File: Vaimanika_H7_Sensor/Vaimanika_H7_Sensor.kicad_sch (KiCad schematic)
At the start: 67 parts, among them SW1 TS-1088-AR02016, U1 TCAN334G, U2 STM32H743VITx, U3 NCP163ASN330T1G, U4 MS5611-01BA, U5 ICM-42688-P, U6 ICM-42688-P, U7 W25Q128JVS, U8 RT9080-33GJ5, U9 BMI088, Y1 25 MHz

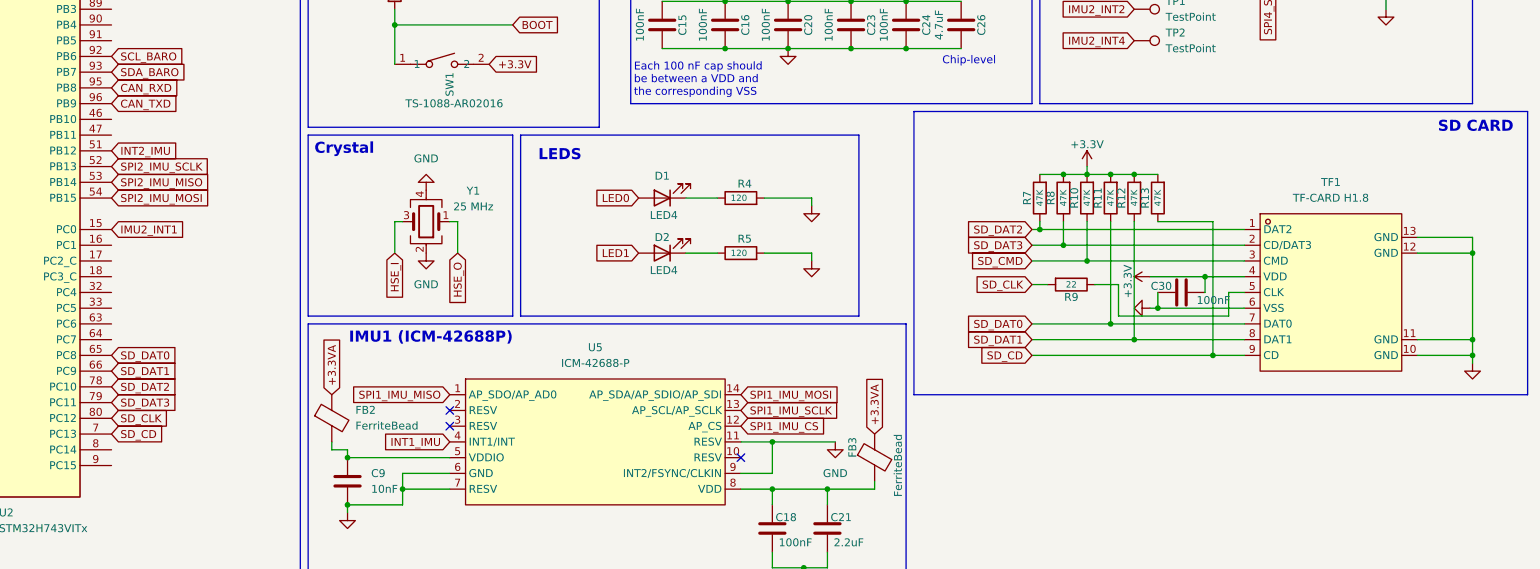
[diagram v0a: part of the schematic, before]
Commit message: 28-03-2025
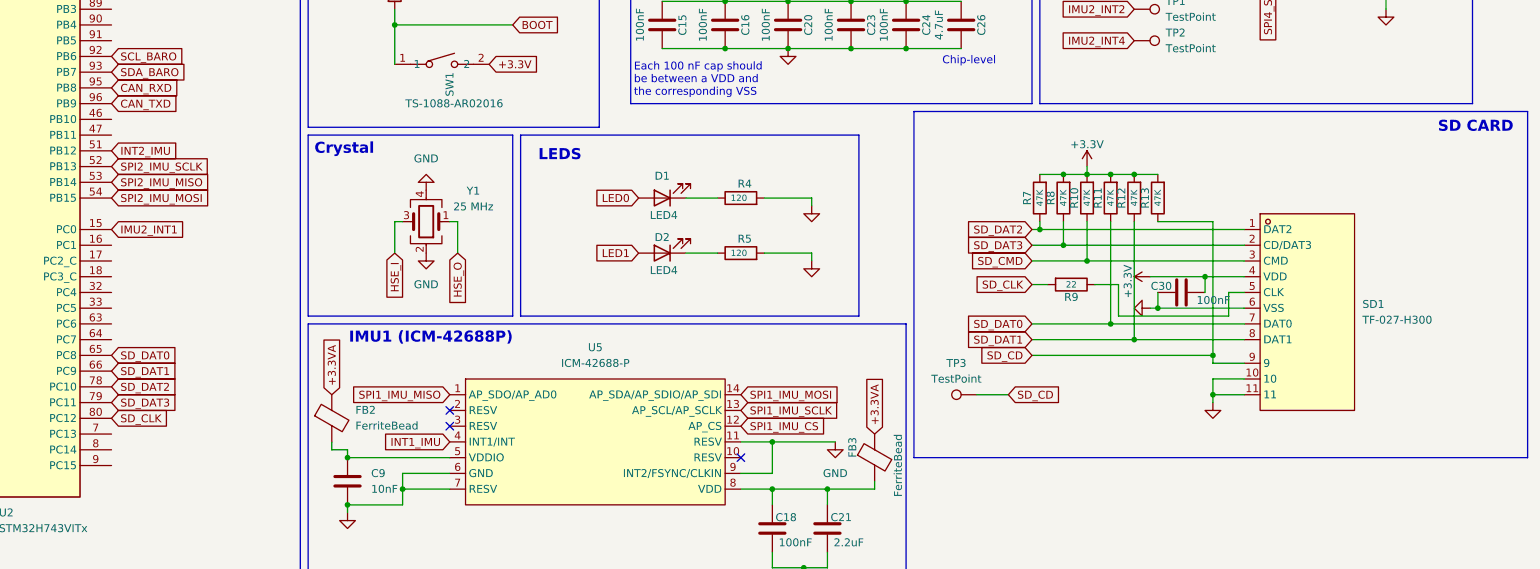
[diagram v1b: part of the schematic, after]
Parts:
- removed TF1: TF-CARD H1.8, New_Library:TF-SMD_TF-CARD-H1.8, symbol New_Library:TF-CARDH1.8
- added SD1: TF-027-H300, New_Library:TF-SMD_HYCW104-TF08-375B, symbol New_Library:TF-027-H300
- added TP3: TestPoint, TestPoint:TestPoint_Pad_D1.0mm, symbol Connector:TestPoint
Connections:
- net +3.3V: now also SD1.4 (VDD)
- net GND: now also SD1.10, SD1.11, SD1.6 (VSS)
- net SD_CD: now also SD1.9, TP3.1; no longer U2.7 (PC13)
- net SD_CMD: now also SD1.3 (CMD)
- net SD_DAT0: now also SD1.7 (DAT0)
- net SD_DAT1: now also SD1.8 (DAT1)
- net SD_DAT2: now also SD1.1 (DAT2)
- net SD_DAT3: now also SD1.2 (CD/DAT3)
- net at R9.1: now also SD1.5 (CLK)

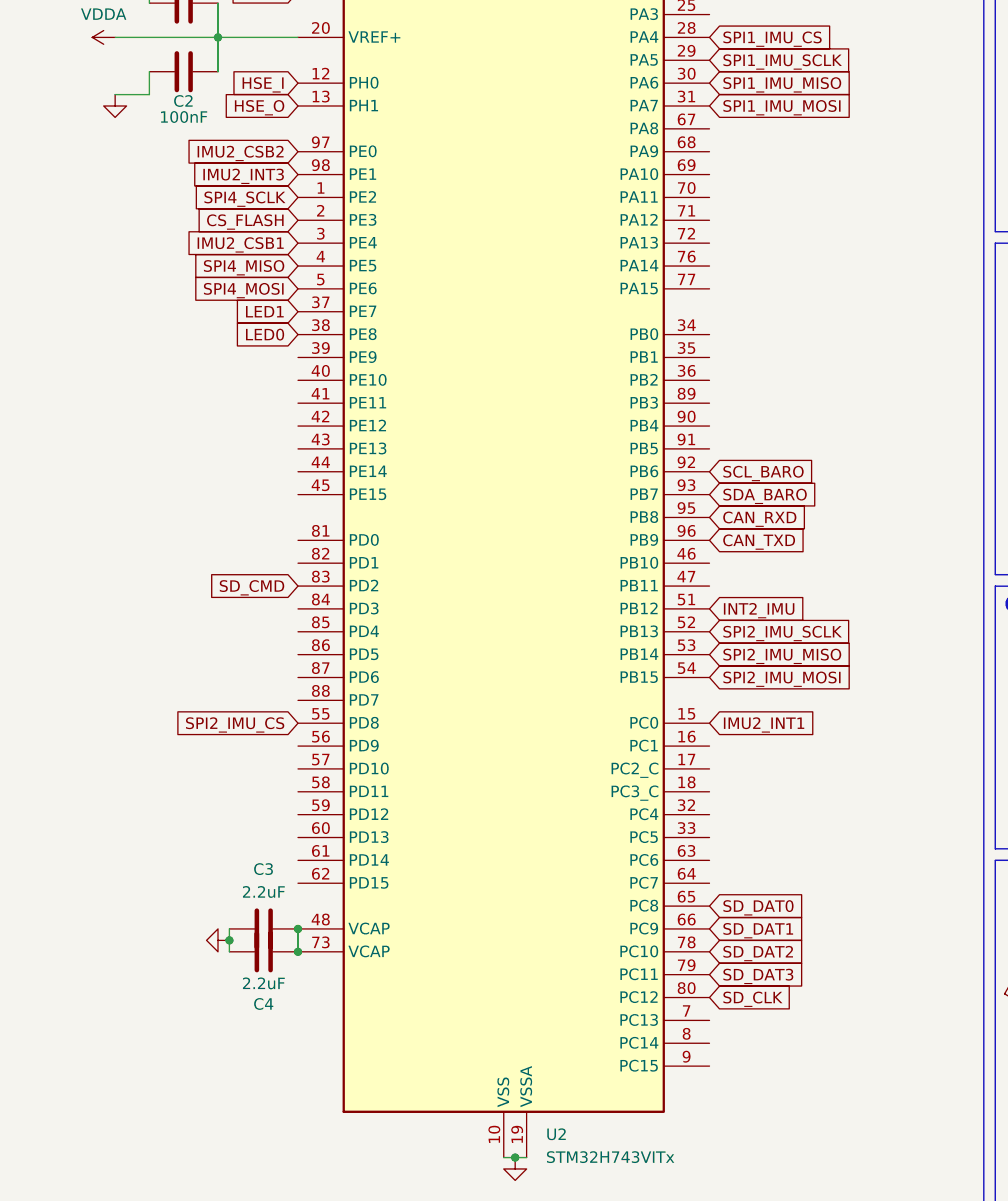
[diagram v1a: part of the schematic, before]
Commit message: 10-04-2026
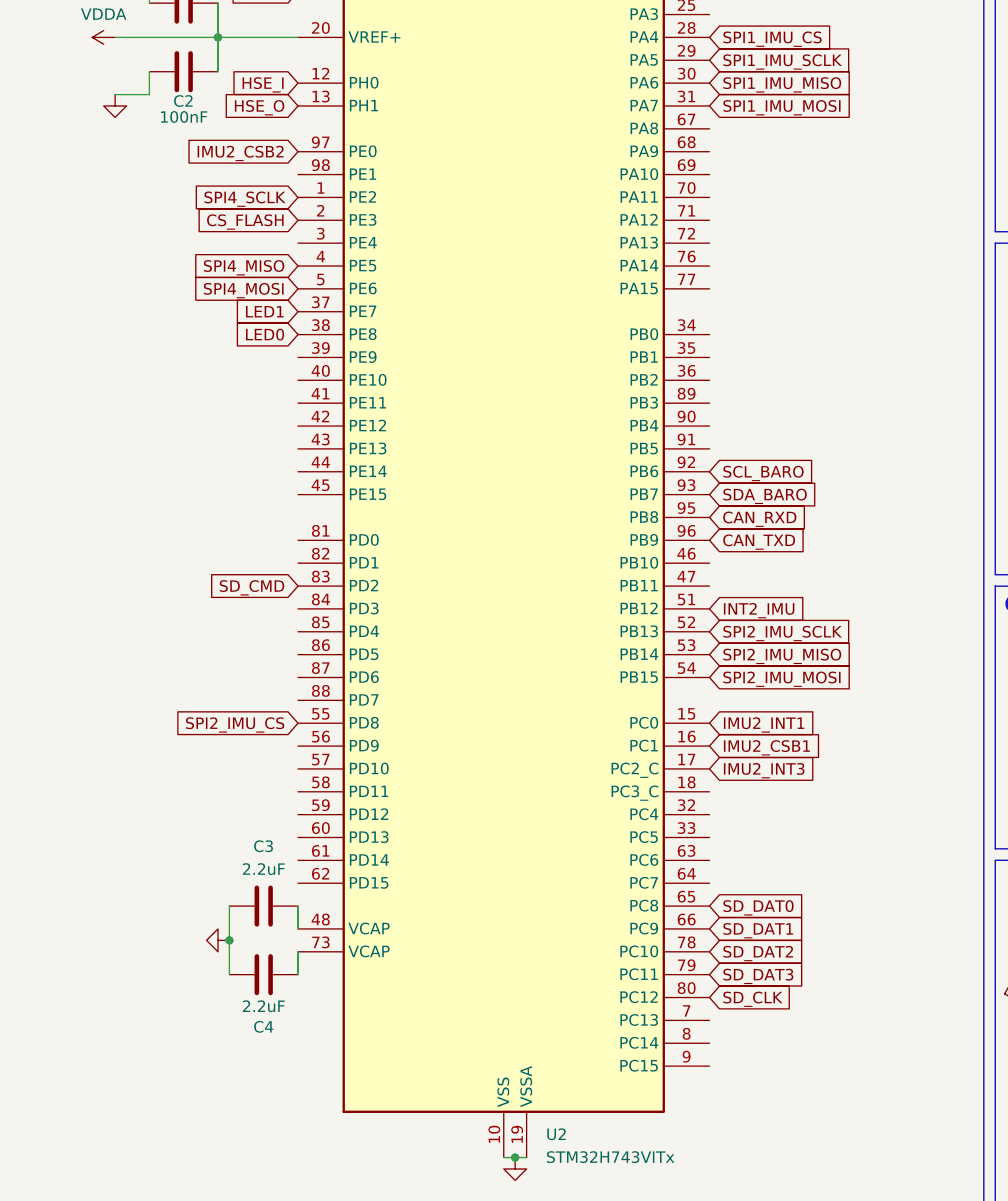
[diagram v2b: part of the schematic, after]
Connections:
- net IMU2_CSB1: now also U2.16 (PC1); no longer U2.3 (PE4)
- net IMU2_INT3: now also U2.17 (PC2_C); no longer U2.98 (PE1)
- net at C3.2, U2.48 (VCAP): no longer C4.2, U2.73 (VCAP)
- new net: C4.2, U2.73 (VCAP)
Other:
- moved on the sheet: C3, C4
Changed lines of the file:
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@@
 	)
 	(junction
-		(at 58.42 162.56)
-		(diameter 0)
-		(color 0 0 0 0)
-	)
-	(junction
 		(at 49.53 60.96)
 		(diameter 0)
@@
 	)
 	(junction
-		(at 58.42 160.02)
-		(diameter 0)
-		(color 0 0 0 0)
-	)
-	(junction
 		(at 83.82 40.64)
 		(diameter 0)
@@
 	(wire
 		(pts
-			(xy 50.8 160.02) (xy 50.8 161.29)
+			(xy 50.8 157.48) (xy 50.8 161.29)
 		)
 		(stroke
@@
 	(wire
 		(pts
+			(xy 58.42 162.56) (xy 58.42 165.1)
+		)
+		(stroke
+			(width 0)
+			(type default)
+		)
+	)
+	(wire
+		(pts
 			(xy 259.08 44.45) (xy 262.89 44.45)
 		)
@@
 	(wire
 		(pts
-			(xy 58.42 160.02) (xy 58.42 162.56)
-		)
-		(stroke
-			(width 0)
-			(type default)
-		)
-	)
-	(wire
-		(pts
 			(xy 210.82 189.23) (xy 210.82 191.77)
 		)
@@
 	(wire
 		(pts
-			(xy 50.8 161.29) (xy 50.8 162.56)
+			(xy 50.8 161.29) (xy 50.8 165.1)
 		)
 		(stroke
@@
 		)
 	)
+	(wire
+		(pts
+			(xy 58.42 157.48) (xy 58.42 160.02)
+		)
+		(stroke
+			(width 0)
+			(type default)
+		)
+	)
 	(global_label "CS_FLASH"
 		(shape input)
@@
 	(global_label "IMU2_CSB1"
 		(shape input)
-		(at 58.42 83.82 180)
+		(at 104.14 139.7 0)
 		(fields_autoplaced yes)
 		(effects
@@
 				(size 1.27 1.27)
 			)
-			(justify right)
+			(justify left)
 		)
 		(property "Intersheetrefs" "${INTERSHEET_REFS}"
-			(at 44.912 83.82 0)
+			(at 117.648 139.7 0)
 			(effects
 				(font
 					(size 1.27 1.27)
 				)
-				(justify right)
+				(justify left)
 				(hide yes)
 			)
@@
 	(global_label "IMU2_INT3"
 		(shape input)
-		(at 58.42 76.2 180)
+		(at 104.14 142.24 0)
 		(fields_autoplaced yes)
 		(effects
@@
 				(size 1.27 1.27)
 			)
-			(justify right)
+			(justify left)
 		)
 		(property "Intersheetrefs" "${INTERSHEET_REFS}"
-			(at 45.7586 76.2 0)
+			(at 116.8014 142.24 0)
 			(effects
 				(font
 					(size 1.27 1.27)
 				)
-				(justify right)
+				(justify left)
 				(hide yes)
 			)
@@
 	(symbol
 		(lib_id "Device:C")
-		(at 54.61 160.02 90)
+		(at 54.61 157.48 90)
 		(unit 1)
 		(exclude_from_sim no)
@@
 		(dnp no)
 		(property "Reference" "C3"
-			(at 54.61 153.416 90)
+			(at 54.61 150.876 90)
 			(effects
 				(font
@@
 		)
 		(property "Value" "2.2uF"
-			(at 54.61 155.956 90)
+			(at 54.61 153.416 90)
 			(effects
 				(font
@@
 		)
 		(property "Footprint" "Capacitor_SMD:C_0402_1005Metric"
-			(at 58.42 159.0548 0)
+			(at 58.42 156.5148 0)
 			(effects
 				(font
@@
 		)
 		(property "Datasheet" "~"
-			(at 54.61 160.02 0)
+			(at 54.61 157.48 0)
 			(effects
 				(font
@@
 		)
 		(property "Description" "Unpolarized capacitor"
-			(at 54.61 160.02 0)
+			(at 54.61 157.48 0)
 			(effects
 				(font
@@
 		)
 		(property "LCSC" "C20539421"
-			(at 54.61 160.02 90)
+			(at 54.61 157.48 90)
 			(effects
 				(font
@@
 		)
 		(property "BOARD" "SENSOR"
-			(at 54.61 160.02 90)
+			(at 54.61 157.48 90)
 			(effects
 				(font
@@
 	(symbol
 		(lib_id "Device:C")
-		(at 54.61 162.56 90)
+		(at 54.61 165.1 90)
 		(unit 1)
 		(exclude_from_sim no)
@@
 		(dnp no)
 		(property "Reference" "C4"
-			(at 54.61 168.402 90)
+			(at 54.61 170.942 90)
 			(effects
 				(font
@@
 		)
 		(property "Value" "2.2uF"
-			(at 54.61 166.116 90)
+			(at 54.61 168.656 90)
 			(effects
 				(font
@@
 		)
 		(property "Footprint" "Capacitor_SMD:C_0402_1005Metric"
-			(at 58.42 161.5948 0)
+			(at 58.42 164.1348 0)
 			(effects
 				(font
@@
 		)
 		(property "Datasheet" "~"
-			(at 54.61 162.56 0)
+			(at 54.61 165.1 0)
 			(effects
 				(font
@@
 		)
 		(property "Description" "Unpolarized capacitor"
-			(at 54.61 162.56 0)
+			(at 54.61 165.1 0)
 			(effects
 				(font
@@
 		)
 		(property "LCSC" "C20539421"
-			(at 54.61 162.56 90)
+			(at 54.61 165.1 90)
 			(effects
 				(font
@@
 		)
 		(property "BOARD" "SENSOR"
-			(at 54.61 162.56 90)
+			(at 54.61 165.1 90)
 			(effects
 				(font

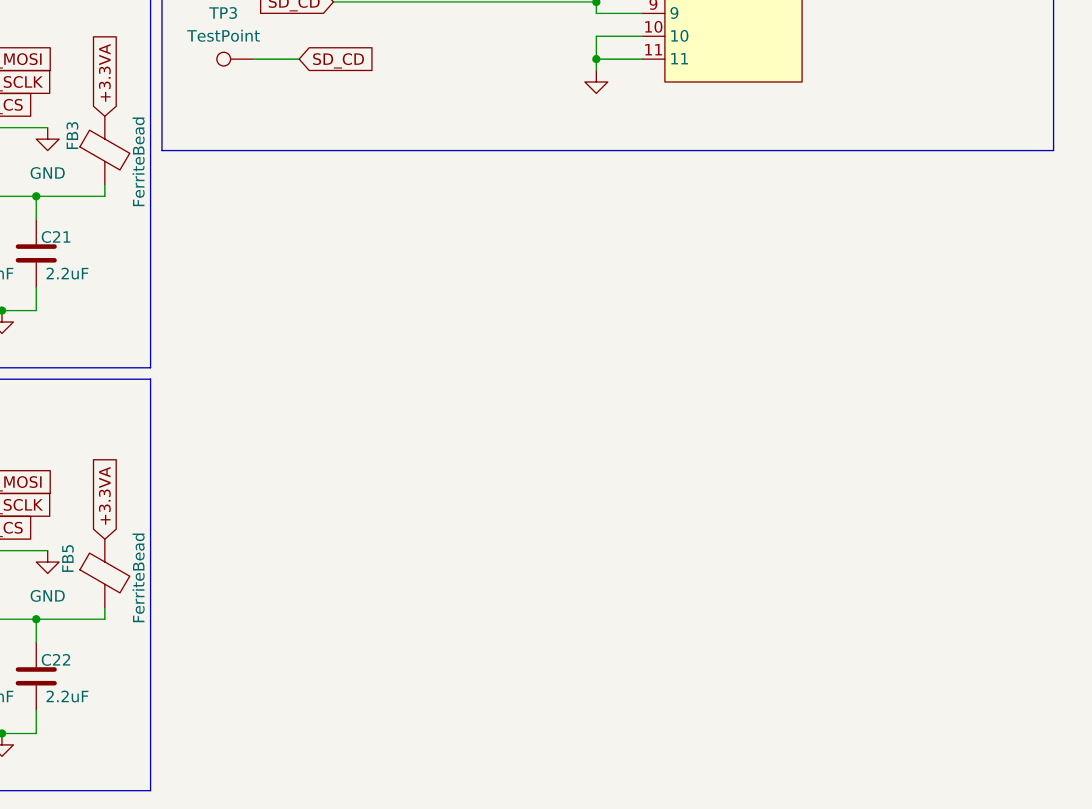
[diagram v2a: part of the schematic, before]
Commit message: 15-04-2026
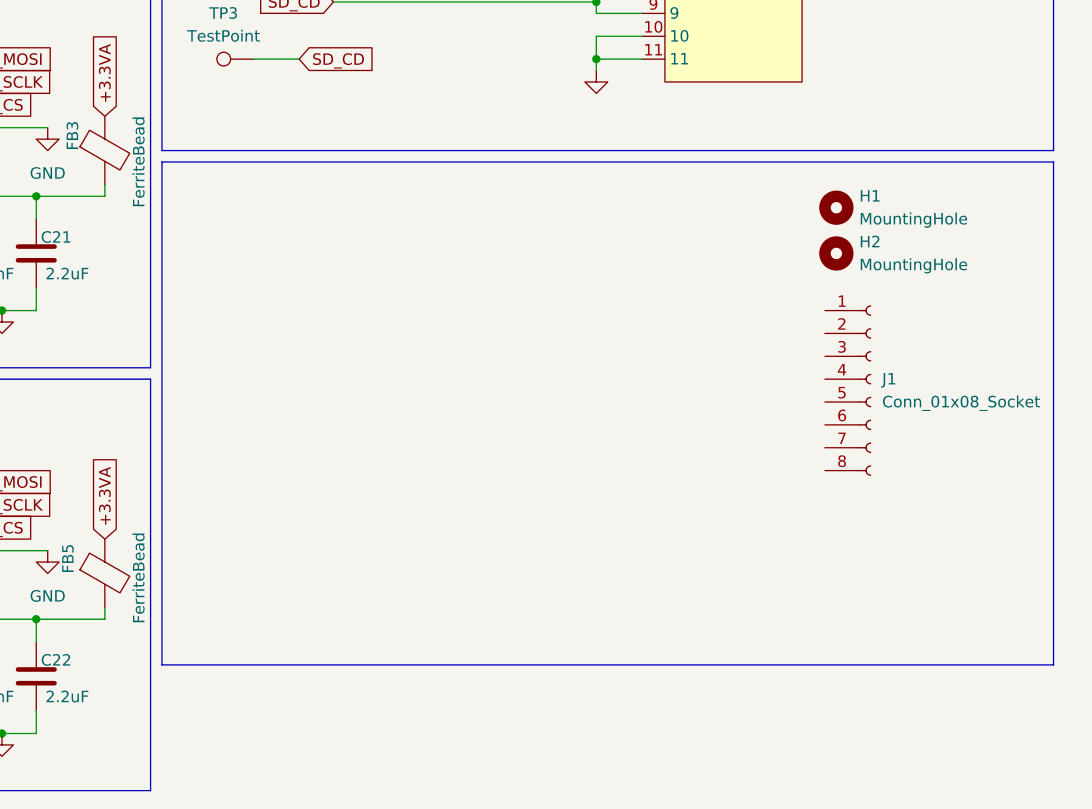
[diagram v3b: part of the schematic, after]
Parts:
- added H1, H2: MountingHole, MountingHole:MountingHole_2.7mm_M2.5_DIN965, symbol Mechanical:MountingHole
- added J1: Conn_01x08_Socket, symbol Connector:Conn_01x08_Socket
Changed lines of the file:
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@@
 	(text_box ""
 		(exclude_from_sim no)
+		(at 233.68 175.26 0)
+		(size 99.06 55.88)
+		(margins 0.9525 0.9525 0.9525 0.9525)
+		(stroke
+			(width 0)
+			(type solid)
+		)
+		(fill
+			(type none)
+		)
+		(effects
+			(font
+				(size 1.27 1.27)
+			)
+			(justify right top)
+		)
+	)
+	(text_box ""
+		(exclude_from_sim no)
 		(at 170.18 121.92 0)
 		(size 54.61 29.21)
@@
 	)
 	(symbol
+		(lib_id "Mechanical:MountingHole")
+		(at 308.61 180.34 0)
+		(unit 1)
+		(exclude_from_sim no)
+		(in_bom no)
+		(on_board yes)
+		(dnp no)
+		(fields_autoplaced yes)
+		(property "Reference" "H1"
+			(at 311.15 179.0699 0)
+			(effects
+				(font
+					(size 1.27 1.27)
+				)
+				(justify left)
+			)
+		)
+		(property "Value" "MountingHole"
+			(at 311.15 181.6099 0)
+			(effects
+				(font
+					(size 1.27 1.27)
+				)
+				(justify left)
+			)
+		)
+		(property "Footprint" "MountingHole:MountingHole_2.7mm_M2.5_DIN965"
+			(at 308.61 180.34 0)
+			(effects
+				(font
+					(size 1.27 1.27)
+				)
+				(hide yes)
+			)
+		)
+		(property "Datasheet" "~"
+			(at 308.61 180.34 0)
+			(effects
+				(font
+					(size 1.27 1.27)
+				)
+				(hide yes)
+			)
+		)
+		(property "Description" "Mounting Hole without connection"
+			(at 308.61 180.34 0)
+			(effects
+				(font
+					(size 1.27 1.27)
+				)
+				(hide yes)
+			)
+		)
+		(instances
+			(project ""
+				(path "/23770a09-842c-46e7-8c45-82f07b31c15d"
+					(reference "H1")
+					(unit 1)
+				)
+			)
+		)
+	)
+	(symbol
 		(lib_id "Device:R")
 		(at 261.62 132.08 180)
@@
 	)
 	(symbol
+		(lib_id "Mechanical:MountingHole")
+		(at 308.61 185.42 0)
+		(unit 1)
+		(exclude_from_sim no)
+		(in_bom no)
+		(on_board yes)
+		(dnp no)
+		(fields_autoplaced yes)
+		(property "Reference" "H2"
+			(at 311.15 184.1499 0)
+			(effects
+				(font
+					(size 1.27 1.27)
+				)
+				(justify left)
+			)
+		)
+		(property "Value" "MountingHole"
+			(at 311.15 186.6899 0)
+			(effects
+				(font
+					(size 1.27 1.27)
+				)
+				(justify left)
+			)
+		)
+		(property "Footprint" "MountingHole:MountingHole_2.7mm_M2.5_DIN965"
+			(at 308.61 185.42 0)
+			(effects
+				(font
+					(size 1.27 1.27)
+				)
+				(hide yes)
+			)
+		)
+		(property "Datasheet" "~"
+			(at 308.61 185.42 0)
+			(effects
+				(font
+					(size 1.27 1.27)
+				)
+				(hide yes)
+			)
+		)
+		(property "Description" "Mounting Hole without connection"
+			(at 308.61 185.42 0)
+			(effects
+				(font
+					(size 1.27 1.27)
+				)
+				(hide yes)
+			)
+		)
+		(instances
+			(project "Vaimanika_H7_Sensor"
+				(path "/23770a09-842c-46e7-8c45-82f07b31c15d"
+					(reference "H2")
+					(unit 1)
+				)
+			)
+		)
+	)
+	(symbol
 		(lib_id "power:+3.3V")
 		(at 213.36 100.33 0)
@@
 					(unit 1)
 				)
+			)
+		)
+	)
+	(symbol
+		(lib_id "Connector:Conn_01x08_Socket")
+		(at 312.42 199.39 0)
+		(unit 1)
+		(exclude_from_sim no)
+		(in_bom yes)
+		(on_board yes)
+		(dnp no)
+		(fields_autoplaced yes)
+		(property "Reference" "J1"
+			(at 313.69 199.3899 0)
+			(effects
+				(font
+					(size 1.27 1.27)
+				)
+				(justify left)
+			)
+		)
+		(property "Value" "Conn_01x08_Socket"
+			(at 313.69 201.9299 0)
+			(effects
+				(font
+					(size 1.27 1.27)
+				)
+				(justify left)
+			)
+		)
+		(property "Footprint" ""
+			(at 312.42 199.39 0)
+			(effects
+				(font
+					(size 1.27 1.27)
+				)
+				(hide yes)
+			)
+		)
+		(property "Datasheet" "~"
+			(at 312.42 199.39 0)
+			(effects
+				(font
+					(size 1.27 1.27)
+				)
+				(hide yes)
+			)
+		)
+		(property "Description" "Generic connector, single row, 01x08, script generated"
+			(at 312.42 199.39 0)
+			(effects
+				(font
+					(size 1.27 1.27)
+				)
+				(hide yes)
+			)
+		)
+		(pin "3"
+		)
+		(pin "7"
+		)
+		(pin "1"
+		)
+		(pin "2"
+		)
+		(pin "5"
+		)
+		(pin "6"
+		)
+		(pin "4"
+		)
+		(pin "8"
+		)
+		(instances
+			(project ""
+				(path "/23770a09-842c-46e7-8c45-82f07b31c15d"
+					(reference "J1")
+					(unit 1)
+				)
